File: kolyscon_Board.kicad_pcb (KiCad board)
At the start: 2 copper layers, 47 parts, among them J1 Conn_01x04, Q1 HL2302, Q10 HL2302, Q11 HL2302, Q2 HL2302, Q3 HL2302, Q4 HL2302, Q5 HL2302, Q6 HL2302, Q7 HL2302, Q8 HL2302, Q9 HL2302, U1 74HC595, U2 74HC595

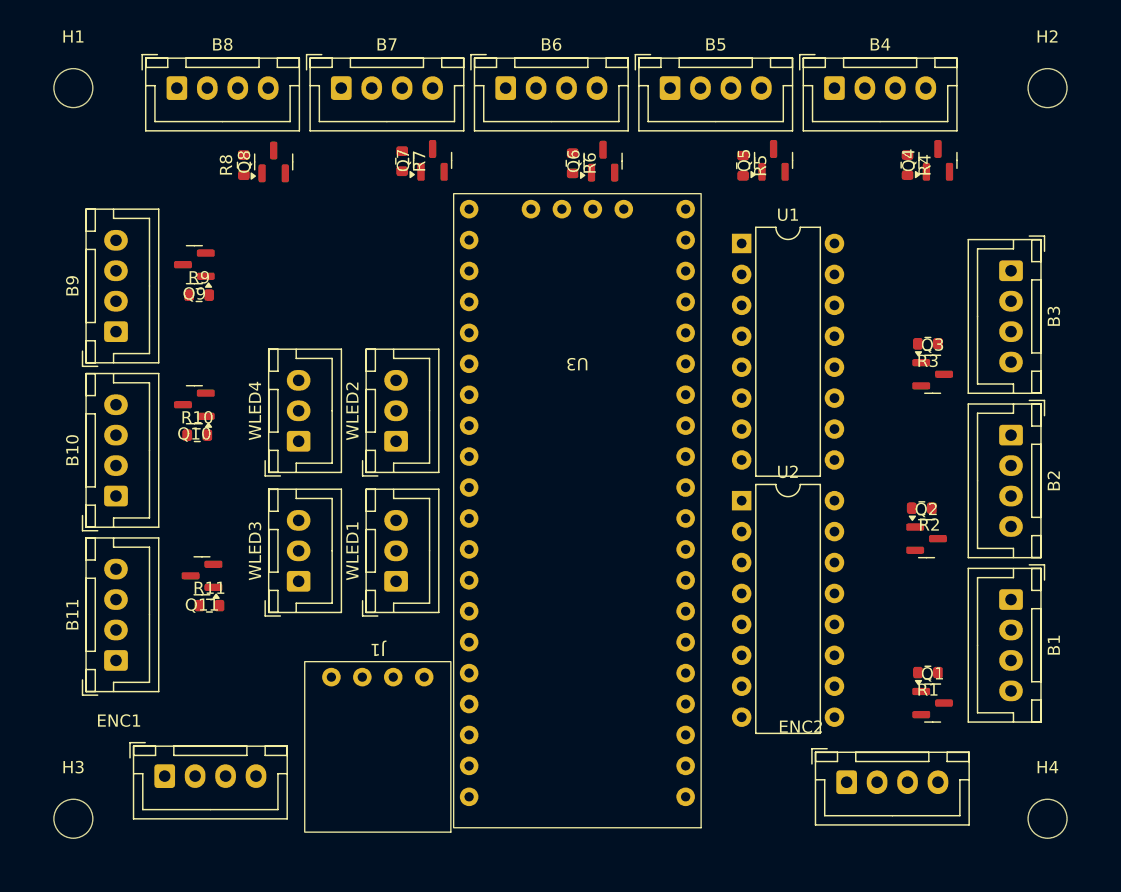
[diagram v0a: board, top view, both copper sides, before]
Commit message: -Routing
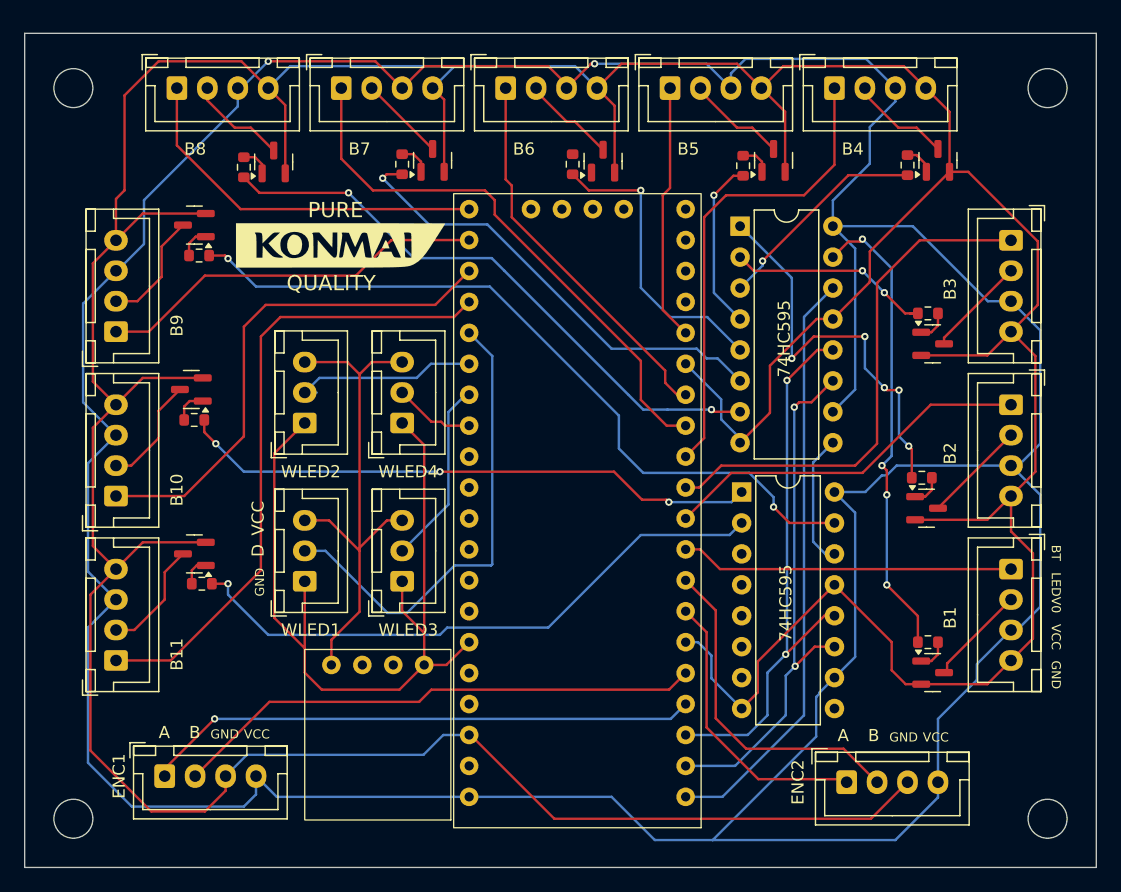
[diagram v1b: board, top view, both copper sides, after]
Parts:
- added G***: LOGO, kolyscon_Board_Footprints:konmai, F.Cu at (92.0, 83.0)
- Q1, Q10, Q11, Q2, Q3, Q4, Q5, Q6, Q7, Q8, Q9: value HL2302 -> ~
- R1, R10, R11, R2, R3, R4, R5, R6, R7, R8, R9: value R -> R1k
- moved WLED4 8.63 mm to (97.0, 97.5)
- moved WLED3 8.50 mm to (97.0, 110.5)
- moved WLED2 7.65 mm to (89.0, 97.5)
- moved WLED1 7.50 mm to (89.0, 110.5)
- moved Q9 3.25 mm to (79.9, 81.2)
- moved R9 3.25 mm to (80.3, 83.8)
- moved B1 2.50 mm to (147.0, 109.5)
- moved B2 2.50 mm to (147.0, 96.0)
- moved B3 2.50 mm to (147.0, 82.5)
- moved Q1 2.50 mm to (140.6, 118.0)
- moved Q2 2.50 mm to (140.1, 104.5)
- moved Q3 2.50 mm to (140.6, 91.0)
- moved R1 2.50 mm to (140.2, 115.5)
- moved R2 2.50 mm to (139.7, 102.0)
- moved R3 2.50 mm to (140.2, 88.5)
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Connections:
- J1 pad 1: GND_PWR -> GND
- U3 pad 10: /BT_D_6 -> /BT_D_2
- U3 pad 11: /BT_D_7 -> /BT_D_3
- U3 pad 12: /BT_D_8 -> /BT_D_4
- U3 pad 13: /BT_D_9 -> /BT_D_7
- U3 pad 14: /BT_D_10 -> /BT_D_6
- U3 pad 15: unconnected-(U3-GND-Pad15) -> GND
- U3 pad 16: /BT_D_11 -> /BT_D_5
- U3 pad 25: /WLED_1 -> /BT_D_8
- U3 pad 26: /WLED_2 -> /BT_D_9
- U3 pad 27: /WLED_3 -> /BT_D_10
- U3 pad 28: /WLED_4 -> /BT_D_11
- U3 pad 29: /ENC_1_A -> /WLED_1
- U3 pad 30: /ENC_1_B -> /WLED_2
- U3 pad 31: /ENC_2_A -> /WLED_3
- U3 pad 32: /ENC_2_B -> /WLED_4
- U3 pad 4: /BT_D_1 -> /ENC_1_A
- U3 pad 5: /BT_D_2 -> /ENC_1_B
- U3 pad 6: unconnected-(U3-GND-Pad6) -> GND
- U3 pad 7: /BT_D_4 -> /ENC_2_A
- U3 pad 8: /BT_D_3 -> /ENC_2_B
- U3 pad 9: /BT_D_5 -> /BT_D_1
- WLED1 pad 1: GND_PWR -> GND
- WLED2 pad 1: GND_PWR -> GND
- WLED3 pad 1: GND_PWR -> GND
- WLED4 pad 1: GND_PWR -> GND
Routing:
- net GND: track 0.00 -> 486.9 mm
- net +5V: track 0.00 -> 348.2 mm, vias 0 -> 2
- net /BT_L_9: track 0.00 -> 62.5 mm, vias 0 -> 2
- net /BT_D_11: track 0.00 -> 52.4 mm
- net /BT_L_11: track 0.00 -> 49.6 mm, vias 0 -> 1
- net /BT_L_8: track 0.00 -> 48.7 mm, vias 0 -> 2
- net /SHIFTREG_SER: track 0.00 -> 48.6 mm
- net /BT_L_10: track 0.00 -> 48.0 mm, vias 0 -> 3
- net /SHIFTREG_LATCH: track 0.00 -> 45.8 mm, vias 0 -> 2
- net /BT_D_7: track 0.00 -> 45.7 mm
- net /ENC_1_A: track 0.00 -> 45.6 mm, vias 0 -> 1
- net /ENC_1_B: track 0.00 -> 43.8 mm
- net +5V_PWR: track 0.00 -> 43.6 mm
- net /SHIFTREG_CLK: track 0.00 -> 43.5 mm, vias 0 -> 2
- net /BT_D_3: track 0.00 -> 42.9 mm
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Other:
- board outline added: 88 x 68.5 mm
- board text added: "A"
- board text added: "B"
- board text added: "BT"
- board text added: "D"
- board text added: "GND"
- board text added: "LEDV0"
- board text added: "PURE"
- board text added: "QUALITY"
- board text added: "VCC"
